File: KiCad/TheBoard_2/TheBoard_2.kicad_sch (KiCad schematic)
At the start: 26 parts, among them J1 Conn_01x03_Female, J2 Conn_01x03_Female, J3 Conn_01x16_Female, J4 Conn_01x36_Male, J5 Conn_01x16_Female, J6 Conn_01x02_Male, U1 MAX680CSA+T, U2 LM337_TO220

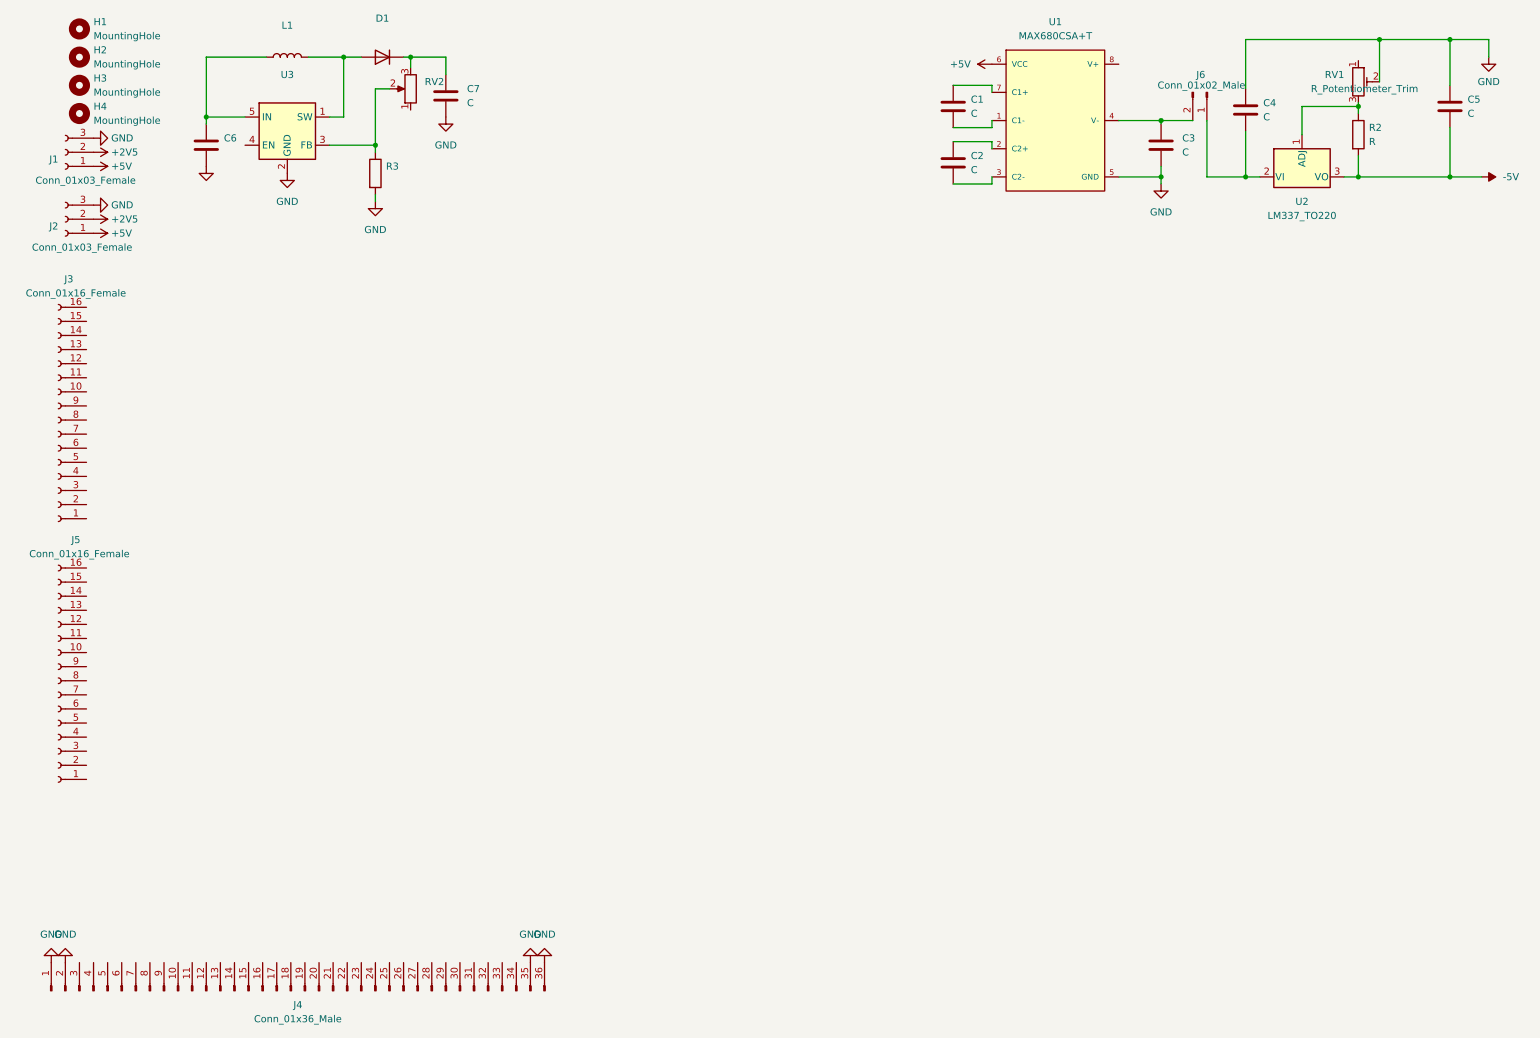
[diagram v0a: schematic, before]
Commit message: Adding battery circuit
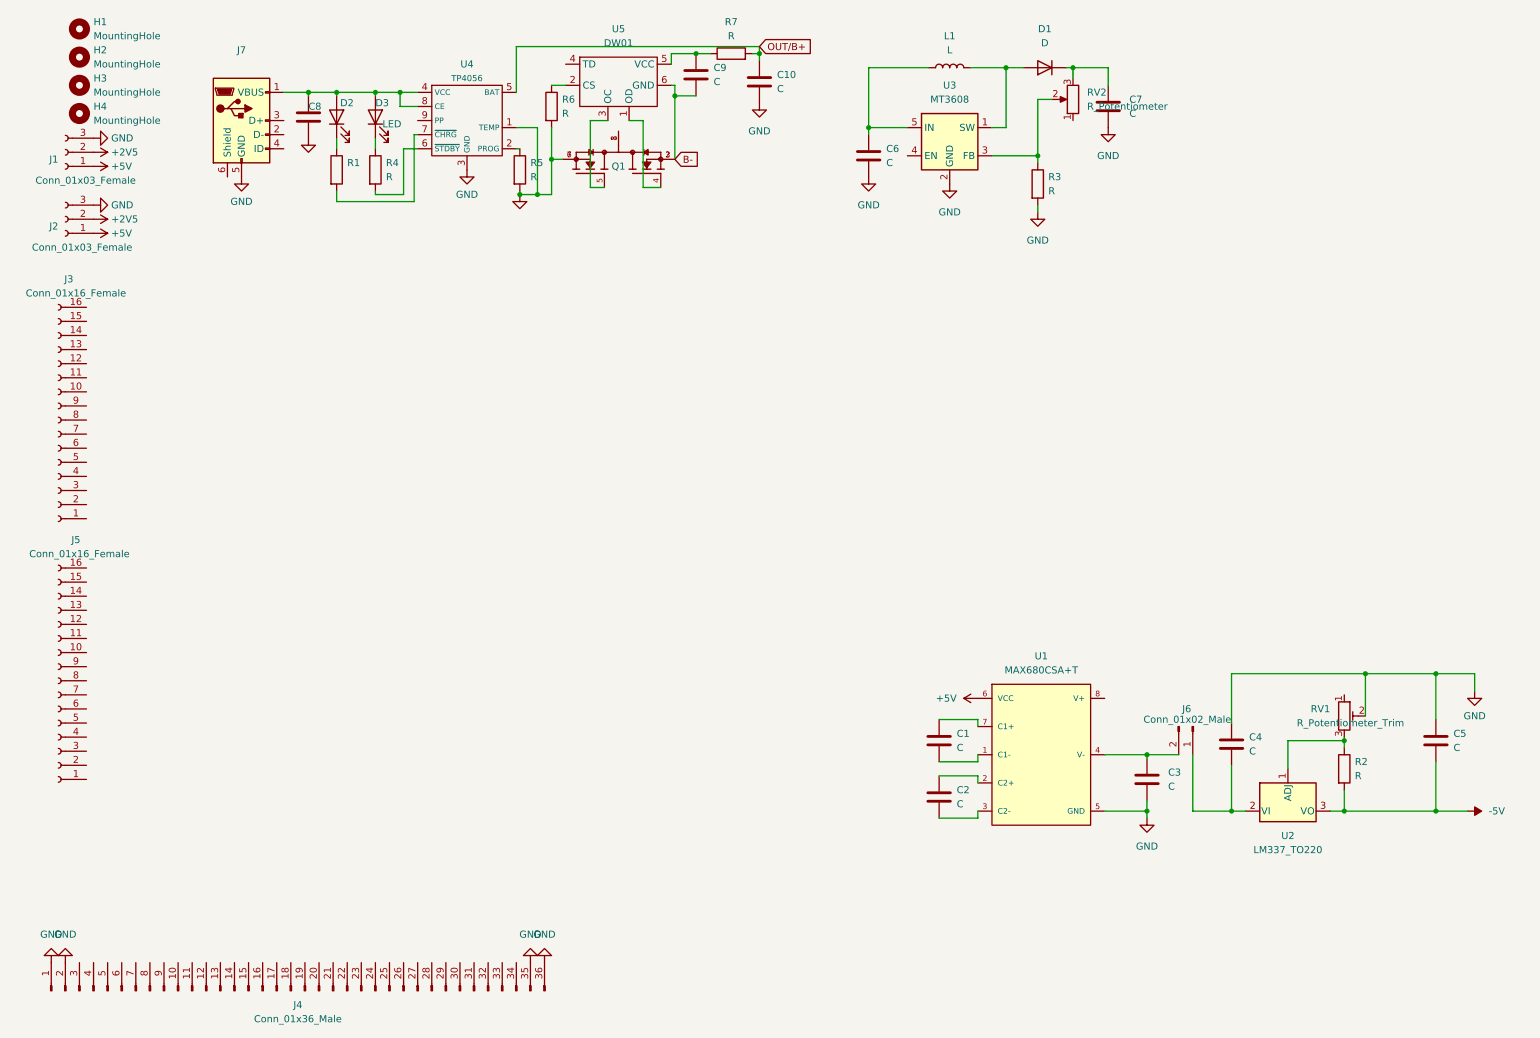
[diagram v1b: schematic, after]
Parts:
- added C10, C9: C, symbol Device:C
- added C8: (no value), symbol Device:C
- added D2: (no value), symbol Device:LED
- added D3: LED, symbol Device:LED
- added J7: (no value), symbol Connector:USB_B_Micro
- added Q1: (no value), symbol FS8205A:FS8205A
- added R1: (no value), symbol Device:R
- added R4, R5, R6, R7: R, symbol Device:R
- added U4: TP4056, Package_SO:SOIC-8-1EP_3.9x4.9mm_P1.27mm_EP2.29x3mm, symbol tp4056:TP4056
- added U5: DW01, Package_TO_SOT_SMD:SOT-23-6_Handsoldering, symbol dw01:DW01
- C6: value (none) -> C; footprint (none) -> Capacitor_SMD:C_1206_3216Metric
- C7: footprint (none) -> Capacitor_SMD:C_1206_3216Metric
- D1: value (none) -> D; footprint (none) -> Diode_SMD:D_SMA
- L1: value (none) -> L; footprint (none) -> Inductor_SMD:L_10.4x10.4_H4.8
- R3: value (none) -> R; footprint (none) -> Resistor_SMD:R_0805_2012Metric
- RV2: value (none) -> R_Potentiometer; footprint (none) -> Potentiometer_THT:Potentiometer_Bourns_3296P_Horizontal
- U3: value (none) -> MT3608; footprint (none) -> Package_TO_SOT_SMD:SOT-23-6
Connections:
- net GND: now also C10.2, C8.2, J7.5 (GND), Q1.6, Q1.7, R5.2, R6.2, U4.1 (TEMP), U4.3 (GND)
- new net: C8.1, D2.2 (A), D3.2 (A), J7.1 (VBUS), U4.4 (VCC), U4.8 (CE)
- new net: Q1.4, U5.1 (OD)
- new net: R6.1, U5.2 (CS)
- new net: Q1.5, U5.3 (OC)
- new net: C9.1, R7.1, U5.5 (VCC)
- new net: D2.1 (K), R1.1
- new net: Q1.1, Q1.8
- new net: D3.1 (K), R4.1
- new net: R5.1, U4.2 (PROG)
- new net: R4.2, U4.6 (~{STDBY})
- new net: R1.2, U4.7 (~{CHRG})
- new net B-: C9.2, Q1.2, Q1.3, U5.6 (GND)
- new net OUT/B+: C10.1, R7.2, U4.5 (BAT)
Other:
- moved on the sheet: C1, C2, C3, C4, C5, C6, C7, D1, J6, L1, R2, R3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
